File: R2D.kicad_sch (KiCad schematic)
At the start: 8 parts, among them Q1 IRF9540N, U1 LM311, U2 7408, U3 74AUC2G02, U4 74AHC1G08, U5 74AUC2G04

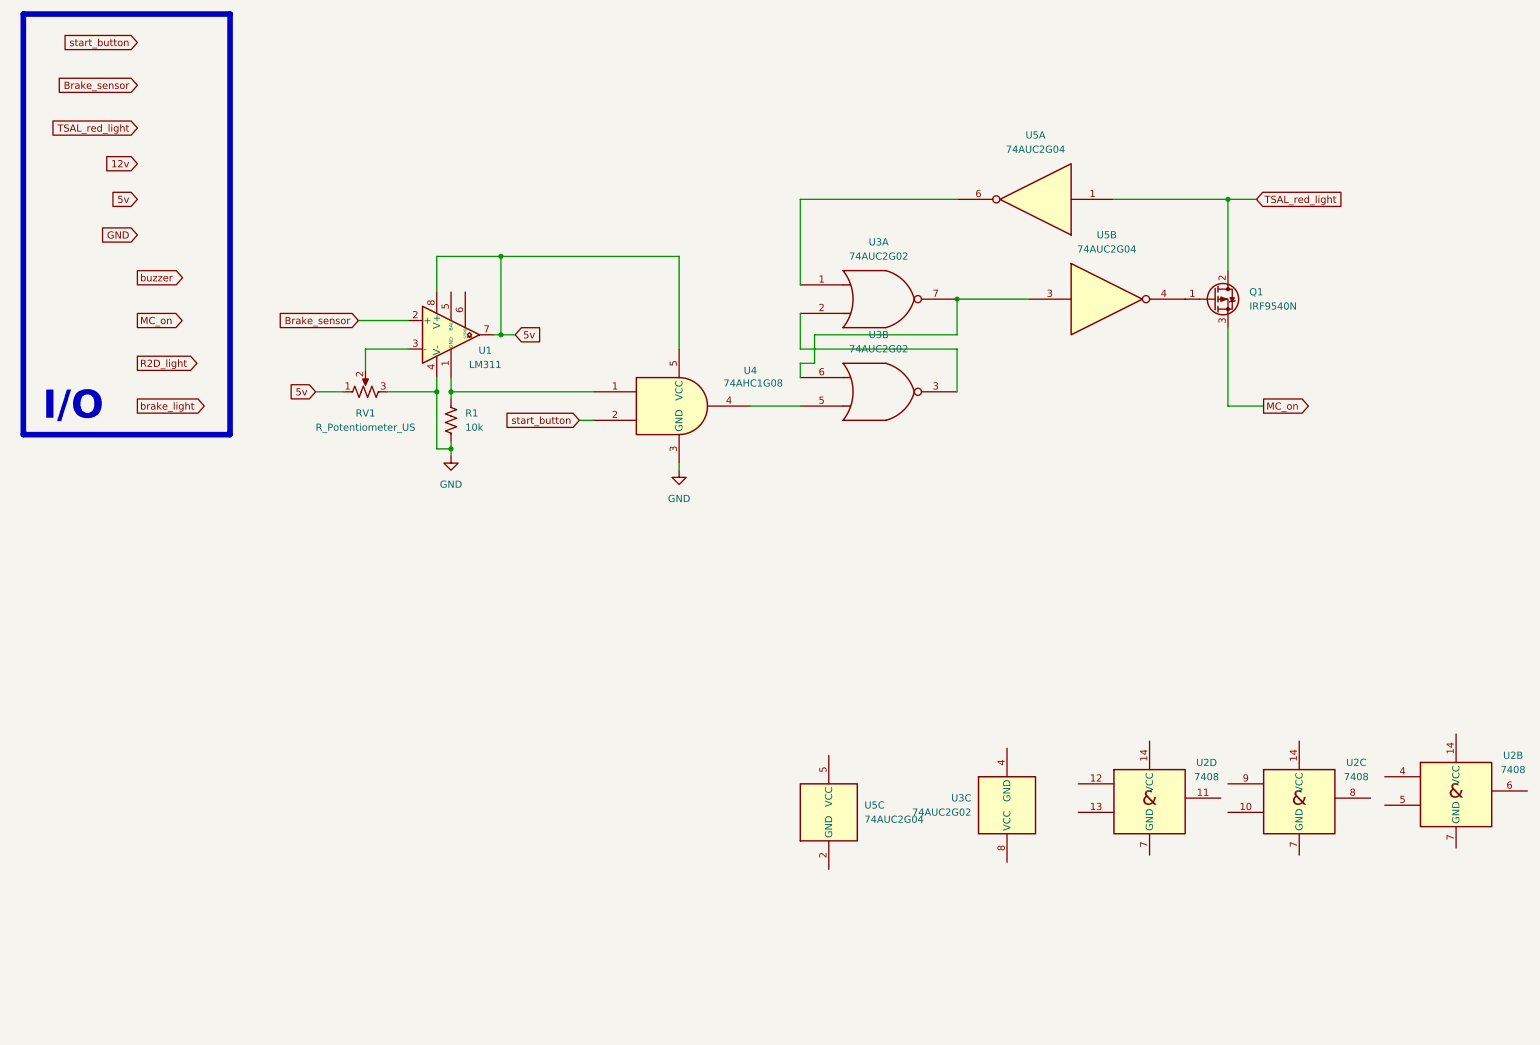
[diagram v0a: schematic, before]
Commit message: update
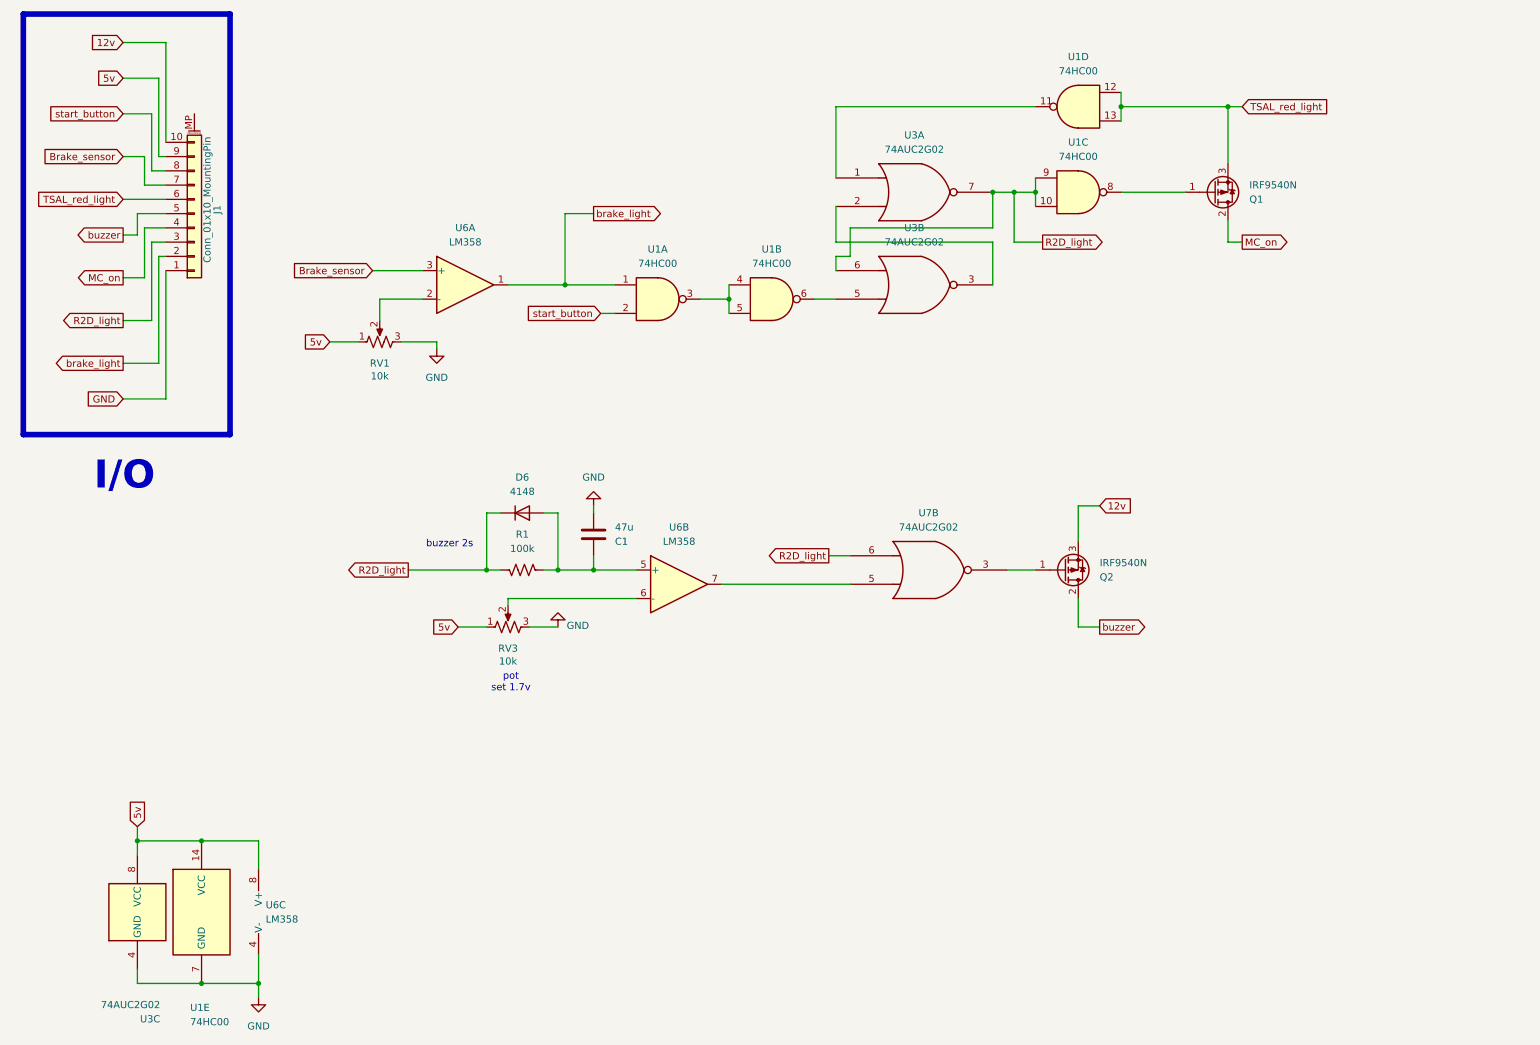
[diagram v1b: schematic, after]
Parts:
- removed U1: LM311, symbol Comparator:LM311
- removed U2: 7408, symbol 74xx_IEEE:7408
- removed U4: 74AHC1G08, symbol 74xGxx:74AHC1G08
- removed U5: 74AUC2G04, symbol 74xGxx:74AUC2G04
- added C1: 47u, Capacitor_THT:CP_Radial_D4.0mm_P2.00mm, symbol Device:C
- added D6: 4148, Diode_THT:D_DO-41_SOD81_P7.62mm_Horizontal, symbol Device:D
- added J1: Conn_01x10_MountingPin, Connector_PinHeader_2.54mm:PinHeader_1x10_P2.54mm_Vertical, symbol Connector_Generic_MountingPin:Conn_01x10_MountingPin
- added Q2: IRF9540N, Package_TO_SOT_THT:TO-220-3_Vertical, symbol Transistor_FET:IRF9540N
- added RV3: 10k, Potentiometer_THT:Potentiometer_Bourns_3339H_Vertical, symbol Device:R_Potentiometer_US
- added U1: 74HC00, Package_DIP:DIP-14_W7.62mm, symbol 74xx:74HC00
- added U6: LM358, Package_DIP:DIP-8_W7.62mm_Socket, symbol Amplifier_Operational:LM358
- added U7: 74AUC2G02, Package_DIP:DIP-14_W7.62mm, symbol 74xGxx:74AUC2G02
- R1: value 10k -> 100k; footprint (none) -> Resistor_THT:R_Axial_DIN0204_L3.6mm_D1.6mm_P7.62mm_Horizontal
- RV1: value R_Potentiometer_US -> 10k; footprint (none) -> Potentiometer_THT:Potentiometer_Bourns_3339H_Vertical
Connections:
- net 12v: now also J1.10 (Pin_10), Q2.3 (S)
- net 5v: now also U3.8 (VCC), J1.9 (Pin_9), RV3.1, U1.14 (VCC), U6.8 (V+)
- net Brake_sensor: now also J1.7 (Pin_7), U6.3 (+)
- net GND: now also U3.4 (GND), C1.2, J1.1 (Pin_1), RV3.3, U1.7 (GND), U6.4 (V-); no longer R1.2
- net MC_on: now also Q1.2 (D), J1.4 (Pin_4); no longer Q1.3 (S)
- net R2D_light: now also R1.2, U3.6, U3.7, D6.1 (K), J1.3 (Pin_3), U1.10, U1.9, U7.6
- net TSAL_red_light: now also Q1.3 (S), J1.6 (Pin_6), U1.12, U1.13; no longer Q1.2 (D)
- net brake_light: now also J1.2 (Pin_2), U1.1, U6.1
- net buzzer: now also J1.5 (Pin_5), Q2.2 (D)
- net start_button: now also J1.8 (Pin_8), U1.2
- net at Q1.1 (G): now also U1.8
- net at U3.5: now also U1.6
- net at U3.1: now also U1.11
- net at RV1.2: now also U6.2 (-)
- net at R1.1: now also C1.1, D6.2 (A), U6.5 (+)
- new net: Q2.1 (G), U7.3
- new net: U6.7, U7.5
- new net: U1.3, U1.4, U1.5
- new net: RV3.2, U6.6 (-)
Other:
- note added: "buzzer 2s"
- note added: "pot set 1.7v"
- moved on the sheet: Q1, RV1, U3A, U3B, U3C
